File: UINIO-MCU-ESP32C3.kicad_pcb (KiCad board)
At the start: 2 copper layers, 59.8 x 20.4 mm, 52 parts, among them J1 Conn_01x15_Male, J2 外接串行下载接口, J3 Conn_01x15_Male, SW1 复位按键, SW2 下载按键, U1 ME6211C33M5G-N, U2 W25Q128JVSSIQ, U3 ESP32-C3, U4 CH343P, Y1 40MHz

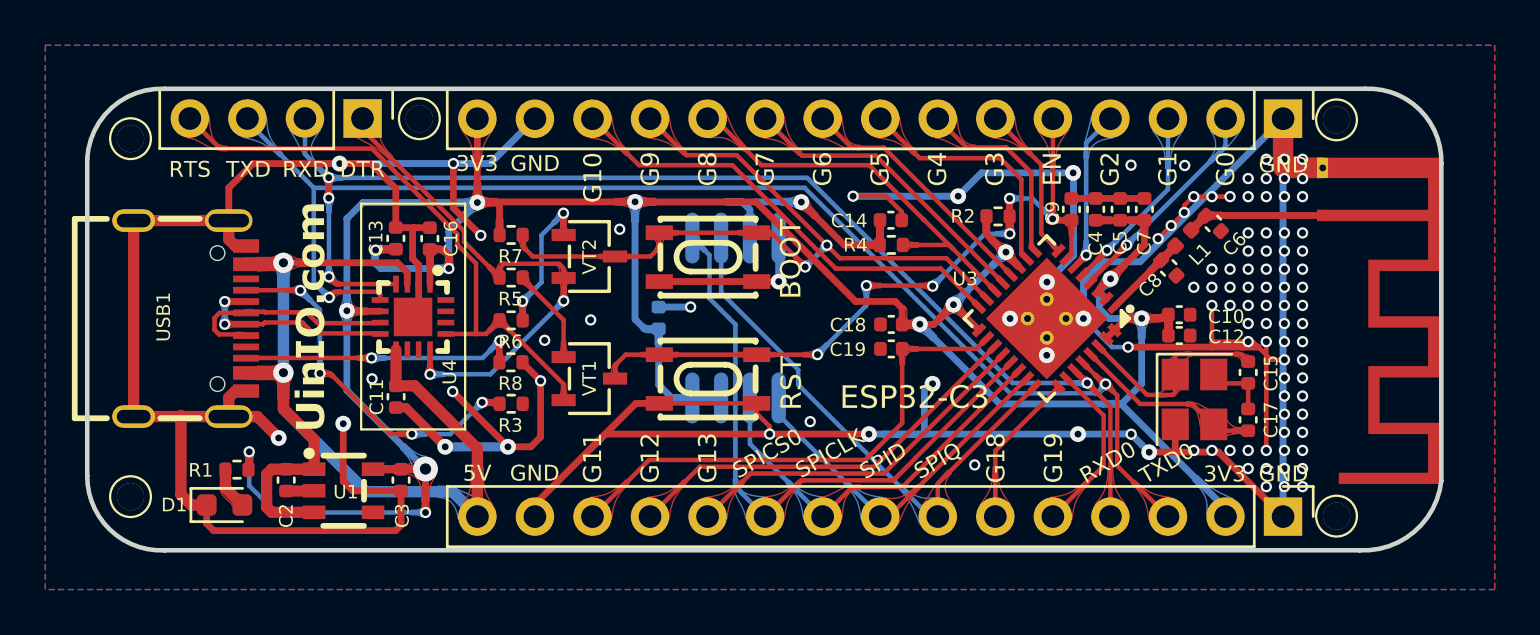
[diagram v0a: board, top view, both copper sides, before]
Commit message: PCB Update.
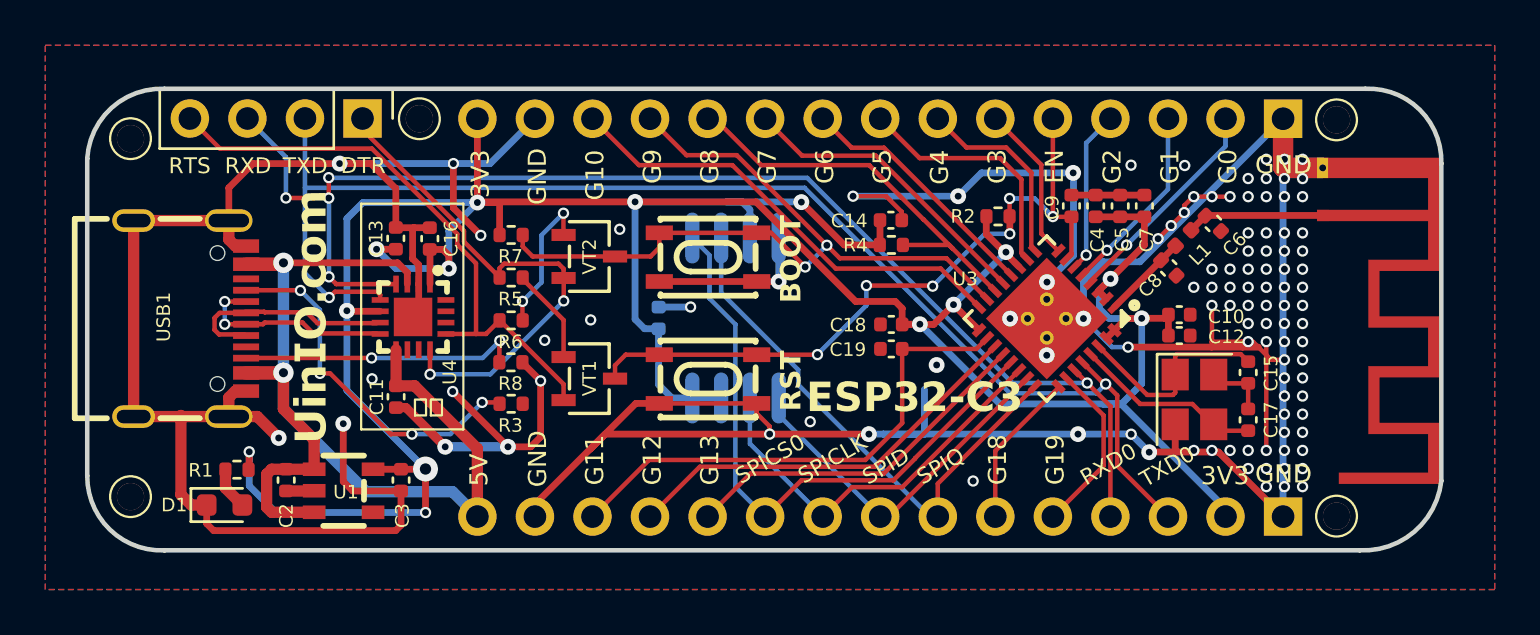
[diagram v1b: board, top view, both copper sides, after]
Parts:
- J1, J3: value Conn_01x15_Male -> Conn_01x15_Pin; moved to B.Cu
- J2: value 外接串行下载接口 -> Conn_01x04_Pin
- moved C4 0.15 mm to (165.5, 98.0)
- moved C5 0.15 mm to (166.6, 98.0)
- moved C7 0.15 mm to (167.6, 98.0)
- moved C9 0.15 mm to (164.4, 98.0)
- turned J1 to 90 degrees
- turned J3 to 90 degrees
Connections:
- J2 pad 2: /U0RXD -> /U0TXD
- J2 pad 3: /U0TXD -> /U0RXD
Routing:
- net /U0RXD: track 54.9 -> 57.9 mm, vias 4 -> 5
- net /U0TXD: track 59.2 -> 58.7 mm
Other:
- board text added: "Version 3.3.0"
- board text added: "可选"
- board text removed: "Version 3.2.0"
